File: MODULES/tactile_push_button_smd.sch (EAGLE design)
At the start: 2 parts

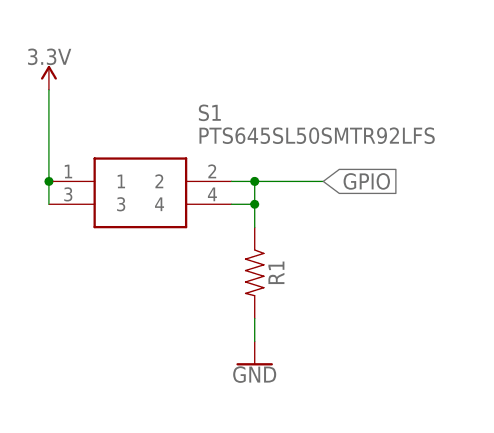
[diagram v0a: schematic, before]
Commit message: Fix board modules
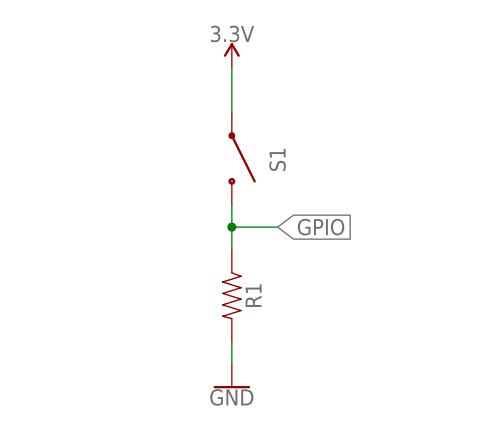
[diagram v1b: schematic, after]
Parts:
- S1: value PTS645SL50SMTR92LFS -> PTS645SL50SMTR92LFS_PTS645SL50SMTR92LFS; device PTS645SL50SMTR92LFS:PTS645SL50SMTR92LFS -> tactile_push_button_smd:PTS645SL50SMTR92LFS_PTS645SL50SMTR92LFS
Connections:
- net 3.3V: no longer S1.3
- net GPIO: no longer S1.4
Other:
- moved on the sheet: R1
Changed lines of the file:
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@@
 </classes>
 <parts>
-<part name="S1" library="PTS645SL50SMTR92LFS" deviceset="PTS645SL50SMTR92LFS" device=""/>
 <part name="R1" library="SparkFun-Resistors" library_urn="urn:adsk.eagle:library:532" deviceset="RESISTOR" device="1206" package3d_urn="urn:adsk.eagle:package:39654/1" value=" "/>
 <part name="SUPPLY1" library="SparkFun-PowerSymbols" library_urn="urn:adsk.eagle:library:530" deviceset="3.3V" device=""/>
 <part name="GND1" library="SparkFun-PowerSymbols" library_urn="urn:adsk.eagle:library:530" deviceset="GND" device=""/>
+<part name="S1" library="tactile_push_button_smd" deviceset="PTS645SL50SMTR92LFS_PTS645SL50SMTR92LFS" device=""/>
 </parts>
 <sheets>
@@
 </plain>
 <instances>
-<instance part="S1" gate="G$1" x="-12.7" y="2.54" smashed="yes">
-<attribute name="NAME" x="3.81" y="10.16" size="1.778" layer="95" align="center-left"/>
-<attribute name="VALUE" x="3.81" y="7.62" size="1.778" layer="96" align="center-left"/>
+<instance part="R1" gate="G$1" x="7.62" y="-10.16" smashed="yes" rot="R270">
+<attribute name="NAME" x="9.144" y="-10.16" size="1.778" layer="95" font="vector" rot="R270" align="bottom-center"/>
+<attribute name="VALUE" x="3.556" y="-10.16" size="1.778" layer="96" font="vector" rot="R270" align="top-center"/>
 </instance>
-<instance part="R1" gate="G$1" x="10.16" y="-7.62" smashed="yes" rot="R270">
-<attribute name="NAME" x="11.684" y="-7.62" size="1.778" layer="95" font="vector" rot="R270" align="bottom-center"/>
-<attribute name="VALUE" x="8.636" y="-7.62" size="1.778" layer="96" font="vector" rot="R270" align="top-center"/>
+<instance part="SUPPLY1" gate="G$1" x="7.62" y="15.24" smashed="yes">
+<attribute name="VALUE" x="7.62" y="18.034" size="1.778" layer="96" align="bottom-center"/>
 </instance>
-<instance part="SUPPLY1" gate="G$1" x="-12.7" y="12.7" smashed="yes">
-<attribute name="VALUE" x="-12.7" y="15.494" size="1.778" layer="96" align="bottom-center"/>
+<instance part="GND1" gate="1" x="7.62" y="-20.32" smashed="yes">
+<attribute name="VALUE" x="7.62" y="-20.574" size="1.778" layer="96" align="top-center"/>
 </instance>
-<instance part="GND1" gate="1" x="10.16" y="-17.78" smashed="yes">
-<attribute name="VALUE" x="10.16" y="-18.034" size="1.778" layer="96" align="top-center"/>
+<instance part="S1" gate="G$1" x="10.16" y="5.08" smashed="yes" rot="R270">
+<attribute name="NAME" x="12.7" y="6.35" size="1.778" layer="95" rot="R270" align="center-left"/>
 </instance>
 </instances>
@@
 <net name="GPIO" class="0">
 <segment>
+<label x="12.7" y="-2.54" size="1.778" layer="95" xref="yes"/>
+<pinref part="R1" gate="G$1" pin="1"/>
 <pinref part="S1" gate="G$1" pin="2"/>
-<wire x1="7.62" y1="2.54" x2="10.16" y2="2.54" width="0.1524" layer="91"/>
-<pinref part="R1" gate="G$1" pin="1"/>
-<wire x1="10.16" y1="2.54" x2="10.16" y2="0" width="0.1524" layer="91"/>
-<pinref part="S1" gate="G$1" pin="4"/>
-<wire x1="10.16" y1="0" x2="10.16" y2="-2.54" width="0.1524" layer="91"/>
-<wire x1="7.62" y1="0" x2="10.16" y2="0" width="0.1524" layer="91"/>
-<junction x="10.16" y="0"/>
-<wire x1="10.16" y1="2.54" x2="17.78" y2="2.54" width="0.1524" layer="91"/>
-<junction x="10.16" y="2.54"/>
-<label x="17.78" y="2.54" size="1.778" layer="95" xref="yes"/>
-</segment>
-</net>
-<net name="3.3V" class="0">
-<segment>
-<pinref part="S1" gate="G$1" pin="3"/>
-<pinref part="S1" gate="G$1" pin="1"/>
-<wire x1="-12.7" y1="0" x2="-12.7" y2="2.54" width="0.1524" layer="91"/>
-<wire x1="-12.7" y1="2.54" x2="-12.7" y2="12.7" width="0.1524" layer="91"/>
-<junction x="-12.7" y="2.54"/>
-<pinref part="SUPPLY1" gate="G$1" pin="3.3V"/>
+<wire x1="7.62" y1="-5.08" x2="7.62" y2="-2.54" width="0.1524" layer="91"/>
+<wire x1="7.62" y1="-2.54" x2="7.62" y2="0" width="0.1524" layer="91"/>
+<wire x1="12.7" y1="-2.54" x2="7.62" y2="-2.54" width="0.1524" layer="91"/>
+<junction x="7.62" y="-2.54"/>
 </segment>
 </net>
@@
 <pinref part="R1" gate="G$1" pin="2"/>
 <pinref part="GND1" gate="1" pin="GND"/>
-<wire x1="10.16" y1="-12.7" x2="10.16" y2="-15.24" width="0.1524" layer="91"/>
+<wire x1="7.62" y1="-15.24" x2="7.62" y2="-17.78" width="0.1524" layer="91"/>
 </segment>
 </net>
+<net name="3.3V" class="0">
+<segment>
+<pinref part="SUPPLY1" gate="G$1" pin="3.3V"/>
+<pinref part="S1" gate="G$1" pin="1"/>
+<wire x1="7.62" y1="10.16" x2="7.62" y2="15.24" width="0.1524" layer="91"/>
+</segment>
+</net>
